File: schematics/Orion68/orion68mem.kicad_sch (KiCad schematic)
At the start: 32 parts, among them J100 Euro96pin, J101B TI9900_8BITS, J13 J100A, J14 J100B, J15 J100C, J16 J100A, J17 J100A, J18 J100A, J19 Conn_02x05_Counter_Clockwise, J20 J101A, J29 ramRom29, J3 ramRom3, J30 rom2Rom5_30, J31 ramRom31, J7 J100A, J8 J100B, J9 J100C, U100A 74HC138, U100B 74HC138, U101A RAM_LOW, U101B RAM_HIGH, U102A RAM_LOW, U102B RAM_HIGH, U103A RAM_LOW, U103B RAM_HIGH, U104A RAM_LOW, U104B RAM_HIGH, U105A RAM_LOW, U105B RAM_HIGH, U18 AT29C512, U23 CY62256-70PC, U29 28C256

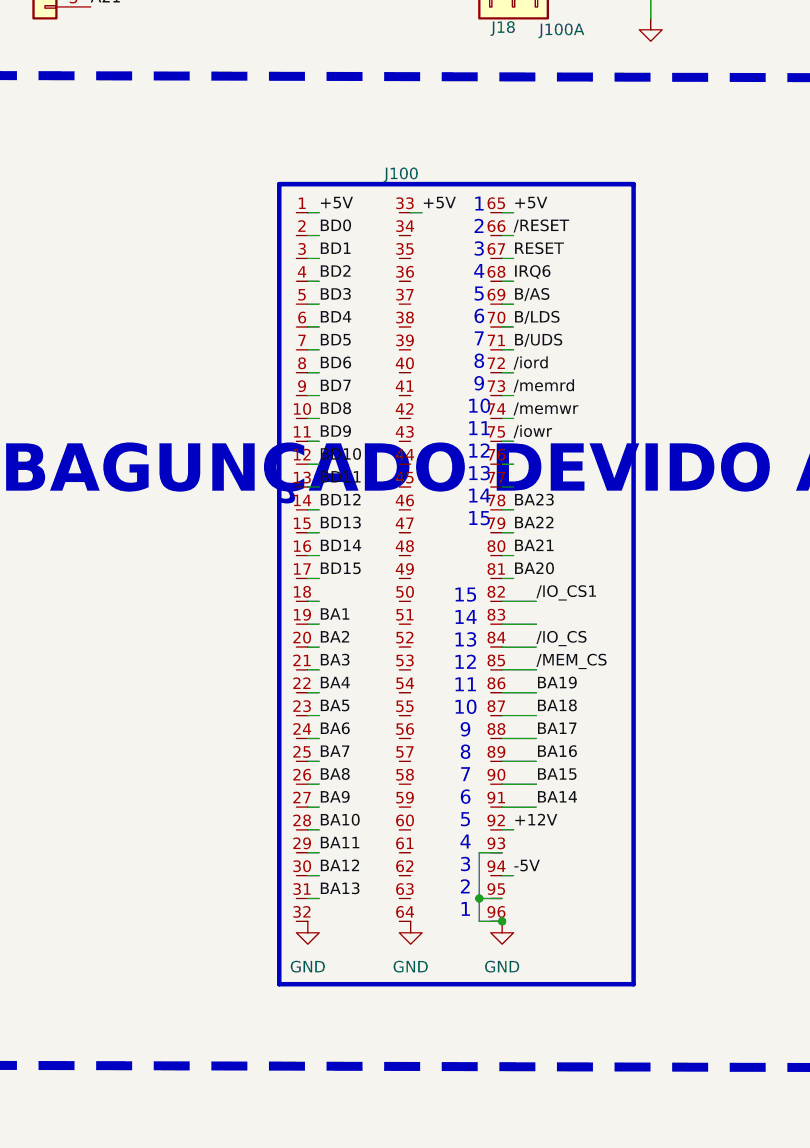
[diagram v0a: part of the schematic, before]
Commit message: update
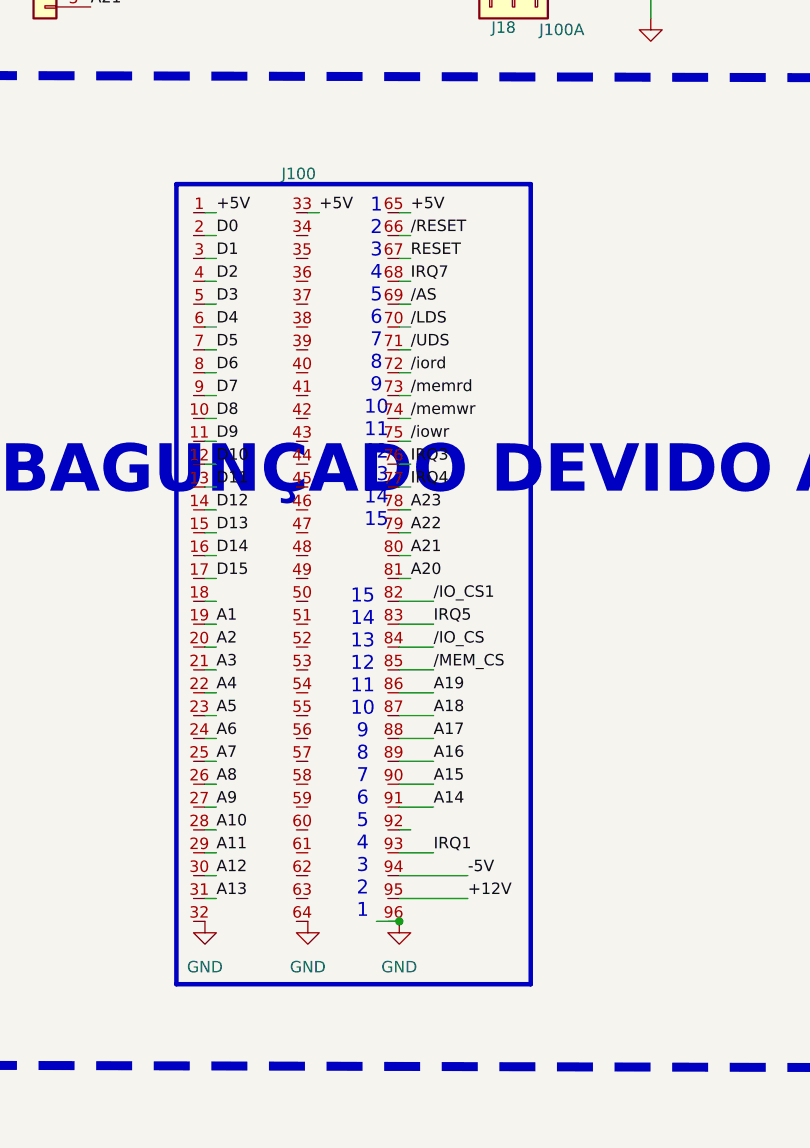
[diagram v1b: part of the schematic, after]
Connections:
- net BA20 is gone; now on net A20: J100.81
- net BA21 is gone; now on net A21: J100.80
- net B/LDS is gone; now on net /LDS: J100.70
- net B/UDS is gone; now on net /UDS: J100.71
- net +12V: now also J100.95; no longer J100.92
- net A16: now also J100.89
- net A19: now also J100.86
- net BA1: no longer J100.19
- net BA10: no longer J100.28
- net BA11: no longer J100.29
- net BA12: no longer J100.30
- net BA13: no longer J100.31
- net BA14: no longer J100.91
- net BA15: no longer J100.90
- net BA16: no longer J100.89
- net BA17: no longer J100.88
- net BA18: no longer J100.87
- net BA19: no longer J100.86
- net BA2: no longer J100.20
- net BA3: no longer J100.21
- net BA4: no longer J100.22
- net BA5: no longer J100.23
- net BA6: no longer J100.24
- net BA7: no longer J100.25
- net BA8: no longer J100.26
- net BA9: no longer J100.27
- net BD0: no longer J100.2
- net BD1: no longer J100.3
- net BD10: no longer J100.12
- net BD11: no longer J100.13
- net BD12: no longer J100.14
- net BD13: no longer J100.15
- net BD14: no longer J100.16
- net BD15: no longer J100.17
- net BD2: no longer J100.4
- net BD3: no longer J100.5
- net BD4: no longer J100.6
- net BD5: no longer J100.7
- net BD6: no longer J100.8
- net BD7: no longer J100.9
- net BD8: no longer J100.10
- net BD9: no longer J100.11
- net GND: no longer J100.93, J100.95
- net IRQ3: now reaches J100.76
- net IRQ4: now reaches J100.77
- net IRQ5: now reaches J100.83
- net BA22 renamed A22
- net BA23 renamed A23
- net B/AS renamed /AS
- net IRQ6 renamed IRQ7
- new net A1: J100.19
- new net A10: J100.28
- new net A11: J100.29
- new net A12: J100.30
- new net A13: J100.31
- new net A14: J100.91
- new net A15: J100.90
- new net A17: J100.88
- new net A18: J100.87
- new net A2: J100.20
- new net A3: J100.21
- new net A4: J100.22
- new net A5: J100.23
- new net A6: J100.24
- new net A7: J100.25
- new net A8: J100.26
- new net A9: J100.27
- new net D0: J100.2
- new net D1: J100.3
- new net D10: J100.12
- new net D11: J100.13
- new net D12: J100.14
- new net D13: J100.15
- new net D14: J100.16
- new net D15: J100.17
- new net D2: J100.4
- new net D3: J100.5
- new net D4: J100.6
- new net D5: J100.7
- new net D6: J100.8
- new net D7: J100.9
- new net D8: J100.10
- new net D9: J100.11
- new net IRQ1: J100.93
